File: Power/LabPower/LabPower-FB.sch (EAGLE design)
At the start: 3 parts

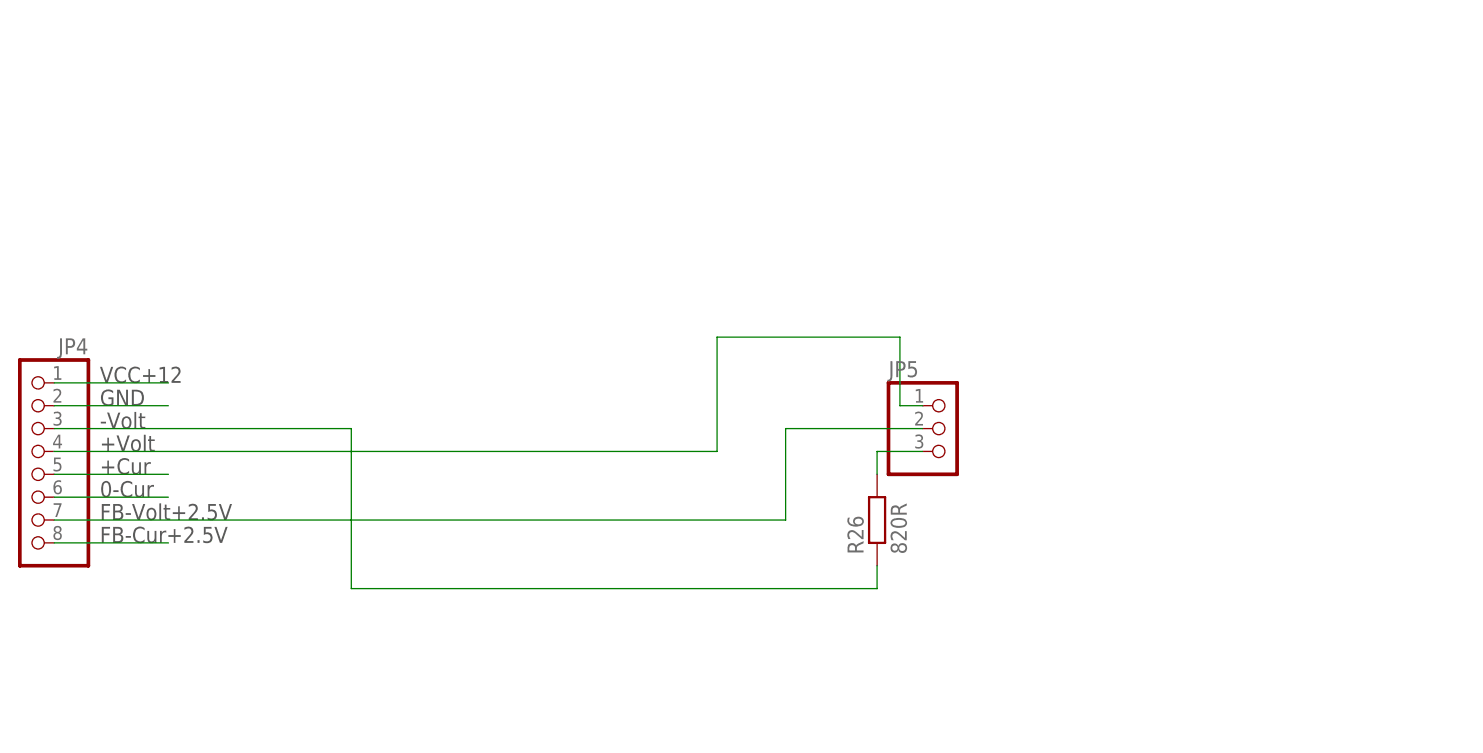
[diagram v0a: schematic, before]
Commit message: _
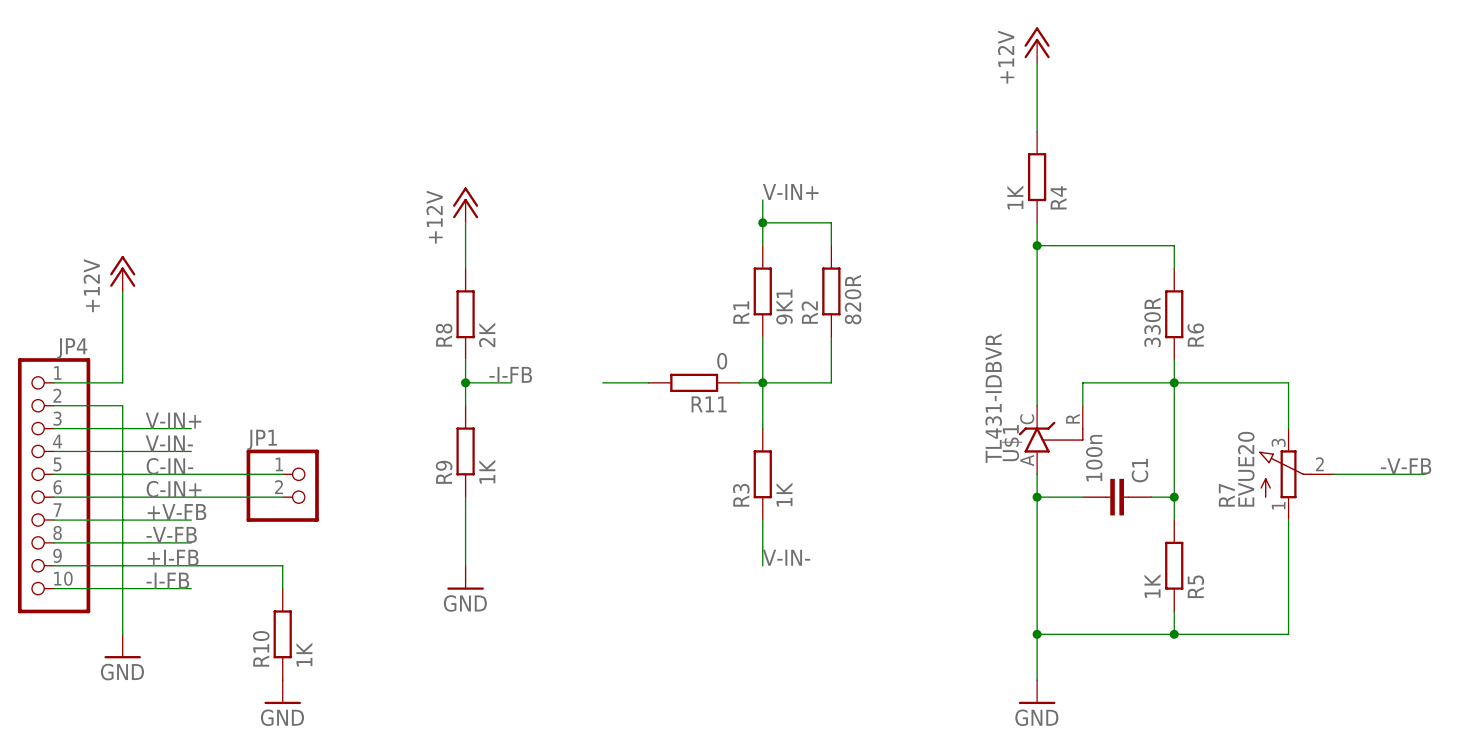
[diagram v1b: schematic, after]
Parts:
- removed JP5: (no value), pinhead:PINHD-1X3
- removed R26: 820R, rcl:R-EU_R0805
- added C1: 100n, rcl:C-EUC0805
- added JP1: (no value), pinhead:PINHD-1X2/90
- added R1: 9K1, rcl:R-EU_R0805
- added R10, R3, R4, R5, R9: 1K, rcl:R-EU_R0805
- added R11: 0, rcl:R-EU_R0805
- added R2: 820R, rcl:R-EU_R0805
- added R6: 330R, rcl:R-EU_R0805
- added R7: EVUE20, pot:EVUE20
- added R8: 2K, rcl:R-EU_R0805
- added U$1: TL431-IDBVR, TL431:TL431-IDBVR
- JP4: device pinhead:PINHD-1X8/90 -> pinhead:PINHD-1X10
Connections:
- removed net N$31: JP4.1
- removed net N$34: JP4.2
- removed net N$37: JP4.3, R26.1
- removed net N$41: JP4.4, JP5.1
- removed net N$42: JP4.5
- removed net N$51: JP4.6
- removed net N$52: JP4.7, JP5.2
- removed net N$53: JP4.8
- removed net N$55: JP5.3, R26.2
- new net +12V: JP4.1, R4.2, R8.2
- new net +I-FB: JP4.9, R10.2
- new net +V-FB: JP4.7, R11.2
- new net -I-FB: JP4.10, R8.1, R9.2
- new net -V-FB: JP4.8, R7.S
- new net C-IN+: JP1.2, JP4.6
- new net C-IN-: JP1.1, JP4.5
- new net GND: C1.2, JP4.2, R10.1, R5.1, R7.A, R9.1, U$1.A
- new net N$1: R4.1, R6.2, U$1.C
- new net N$2: C1.1, R5.2, R6.1, R7.E, U$1.R
- new net N$3: R1.1, R11.1, R2.1, R3.2
- new net V-IN+: JP4.3, R1.2, R2.2
- new net V-IN-: JP4.4, R3.1
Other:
- note removed: "+Cur"
- note removed: "+Volt"
- note removed: "-Volt"
- note removed: "0-Cur"
- note removed: "FB-Cur+2.5V"
- note removed: "FB-Volt+2.5V"
- note removed: "GND"
- note removed: "VCC+12"
